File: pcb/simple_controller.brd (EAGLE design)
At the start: 40 x 52 mm, 66 parts, among them IC1 LD1117S50C, IC2 ST2378E, IC3 MCP1802, IC4 INA196, IC5 INA196, IC6 ATSAMC21G, Q1 24MHz, Q2 32768kHz, T1 NVR4003NT3G, T2 IRF9392PBF, T3 NVR4003NT3G, T4 IRF9392PBF, X1 NANOFIT-2, X11 PINHD-1X2, X2 IGRID-14, X3 IGRID-10, X4 PINHD-1X2, X5 MICRO-LATCH-4, X6 PINHD-1X2, X7 NANOFIT-7, X8 JTAG-EDGE-CON, X9 B3S-1000

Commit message: fixing op amp (iron,tweezer)
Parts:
- C2, C3, C4, C5: value 10µF -> 1µF
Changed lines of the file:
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@@
 <grid distance="0.4" unitdist="mm" unit="mm" style="lines" multiple="1" display="no" altdistance="0.05" altunitdist="mm" altunit="mm"/>
 <layers>
-<layer number="1" name="Top" color="4" fill="1" visible="yes" active="yes"/>
+<layer number="1" name="Top" color="4" fill="1" visible="no" active="yes"/>
 <layer number="2" name="Route2" color="1" fill="3" visible="no" active="no"/>
 <layer number="3" name="Route3" color="4" fill="3" visible="no" active="no"/>
@@
 <layer number="19" name="Unrouted" color="6" fill="1" visible="yes" active="yes"/>
 <layer number="20" name="Dimension" color="24" fill="1" visible="yes" active="yes"/>
-<layer number="21" name="tPlace" color="7" fill="1" visible="yes" active="yes"/>
+<layer number="21" name="tPlace" color="7" fill="1" visible="no" active="yes"/>
 <layer number="22" name="bPlace" color="7" fill="1" visible="yes" active="yes"/>
-<layer number="23" name="tOrigins" color="15" fill="1" visible="yes" active="yes"/>
+<layer number="23" name="tOrigins" color="15" fill="1" visible="no" active="yes"/>
 <layer number="24" name="bOrigins" color="15" fill="1" visible="yes" active="yes"/>
-<layer number="25" name="tNames" color="7" fill="1" visible="yes" active="yes"/>
-<layer number="26" name="bNames" color="7" fill="1" visible="yes" active="yes"/>
+<layer number="25" name="tNames" color="7" fill="1" visible="no" active="yes"/>
+<layer number="26" name="bNames" color="7" fill="1" visible="no" active="yes"/>
 <layer number="27" name="tValues" color="7" fill="1" visible="no" active="yes"/>
 <layer number="28" name="bValues" color="7" fill="1" visible="no" active="yes"/>
@@
 <layer number="37" name="tTest" color="7" fill="1" visible="no" active="yes"/>
 <layer number="38" name="bTest" color="7" fill="1" visible="no" active="yes"/>
-<layer number="39" name="tKeepout" color="4" fill="11" visible="yes" active="yes"/>
-<layer number="40" name="bKeepout" color="1" fill="11" visible="yes" active="yes"/>
-<layer number="41" name="tRestrict" color="4" fill="10" visible="yes" active="yes"/>
-<layer number="42" name="bRestrict" color="1" fill="10" visible="yes" active="yes"/>
-<layer number="43" name="vRestrict" color="2" fill="10" visible="yes" active="yes"/>
+<layer number="39" name="tKeepout" color="4" fill="11" visible="no" active="yes"/>
+<layer number="40" name="bKeepout" color="1" fill="11" visible="no" active="yes"/>
+<layer number="41" name="tRestrict" color="4" fill="10" visible="no" active="yes"/>
+<layer number="42" name="bRestrict" color="1" fill="10" visible="no" active="yes"/>
+<layer number="43" name="vRestrict" color="2" fill="10" visible="no" active="yes"/>
 <layer number="44" name="Drills" color="7" fill="1" visible="no" active="yes"/>
 <layer number="45" name="Holes" color="7" fill="1" visible="yes" active="yes"/>
@@
 <layer number="48" name="Document" color="7" fill="1" visible="no" active="yes"/>
 <layer number="49" name="Reference" color="7" fill="1" visible="no" active="yes"/>
-<layer number="51" name="tDocu" color="7" fill="1" visible="yes" active="yes"/>
+<layer number="51" name="tDocu" color="7" fill="1" visible="no" active="yes"/>
 <layer number="52" name="bDocu" color="7" fill="1" visible="yes" active="yes"/>
 <layer number="88" name="SimResults" color="9" fill="1" visible="no" active="no"/>
@@
 <attribute name="OC_MOUSER" value="667-EEE-FK1E471P" x="8.5" y="22.7" size="1.778" layer="27" rot="R180" display="off"/>
 </element>
-<element name="C2" library="rcl" library_urn="urn:adsk.eagle:library:334" package="C0805" package3d_urn="urn:adsk.eagle:package:23617/2" value="10µF" x="2.6" y="36.65" smashed="yes" rot="MR0">
+<element name="C2" library="rcl" library_urn="urn:adsk.eagle:library:334" package="C0805" package3d_urn="urn:adsk.eagle:package:23617/2" value="1µF" x="2.6" y="36.65" smashed="yes" rot="MR0">
 <attribute name="NAME" x="3.148665625" y="37.7854" size="0.8128" layer="26" rot="MR0"/>
 <attribute name="OC_MOUSER" value="81-GRM21BR61E106MA3L" x="2.6" y="36.65" size="1.778" layer="28" rot="MR0" display="off"/>
@@
 <attribute name="VALUE" x="3.87" y="34.11" size="1.27" layer="28" rot="MR0"/>
 </element>
-<element name="C3" library="rcl" library_urn="urn:adsk.eagle:library:334" package="C0805" package3d_urn="urn:adsk.eagle:package:23617/2" value="10µF" x="3.8" y="23.15" smashed="yes" rot="MR0">
+<element name="C3" library="rcl" library_urn="urn:adsk.eagle:library:334" package="C0805" package3d_urn="urn:adsk.eagle:package:23617/2" value="1µF" x="3.8" y="23.15" smashed="yes" rot="MR0">
 <attribute name="NAME" x="1.8016" y="22.7436" size="0.8128" layer="26" rot="MR0"/>
 <attribute name="OC_MOUSER" value="81-GRM21BR61E106MA3L" x="3.8" y="23.15" size="1.778" layer="28" rot="MR0" display="off"/>
@@
 <attribute name="VALUE" x="5.07" y="20.61" size="1.27" layer="28" rot="MR0"/>
 </element>
-<element name="C4" library="rcl" library_urn="urn:adsk.eagle:library:334" package="C0805" package3d_urn="urn:adsk.eagle:package:23617/2" value="10µF" x="3.8" y="21.1" smashed="yes" rot="MR0">
+<element name="C4" library="rcl" library_urn="urn:adsk.eagle:library:334" package="C0805" package3d_urn="urn:adsk.eagle:package:23617/2" value="1µF" x="3.8" y="21.1" smashed="yes" rot="MR0">
 <attribute name="NAME" x="1.8016" y="20.6936" size="0.8128" layer="26" rot="MR0"/>
 <attribute name="OC_MOUSER" value="81-GRM21BR61E106MA3L" x="3.8" y="21.1" size="1.778" layer="28" rot="MR0" display="off"/>
@@
 <attribute name="VALUE" x="5.07" y="18.56" size="1.27" layer="28" rot="MR0"/>
 </element>
-<element name="C5" library="rcl" library_urn="urn:adsk.eagle:library:334" package="C0805" package3d_urn="urn:adsk.eagle:package:23617/2" value="10µF" x="2.85" y="13.4" smashed="yes" rot="MR180">
+<element name="C5" library="rcl" library_urn="urn:adsk.eagle:library:334" package="C0805" package3d_urn="urn:adsk.eagle:package:23617/2" value="1µF" x="2.85" y="13.4" smashed="yes" rot="MR180">
 <attribute name="NAME" x="1.948928125" y="11.4518" size="0.8128" layer="26" rot="MR0"/>
 <attribute name="OC_MOUSER" value="81-GRM21BR61E106MA3L" x="2.85" y="13.4" size="1.778" layer="28" rot="MR180" display="off"/>

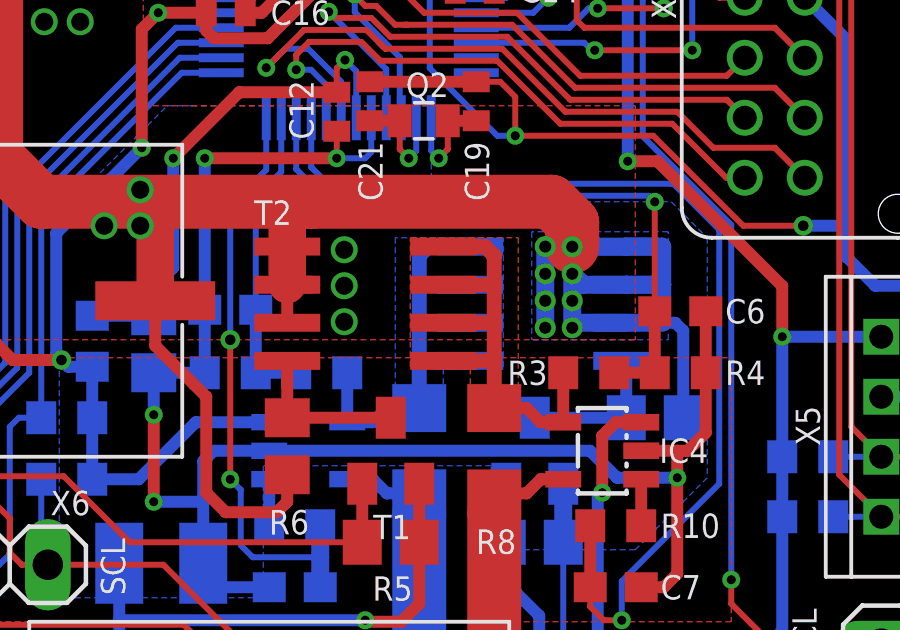
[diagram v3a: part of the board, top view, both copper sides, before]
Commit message: iron drills deleted
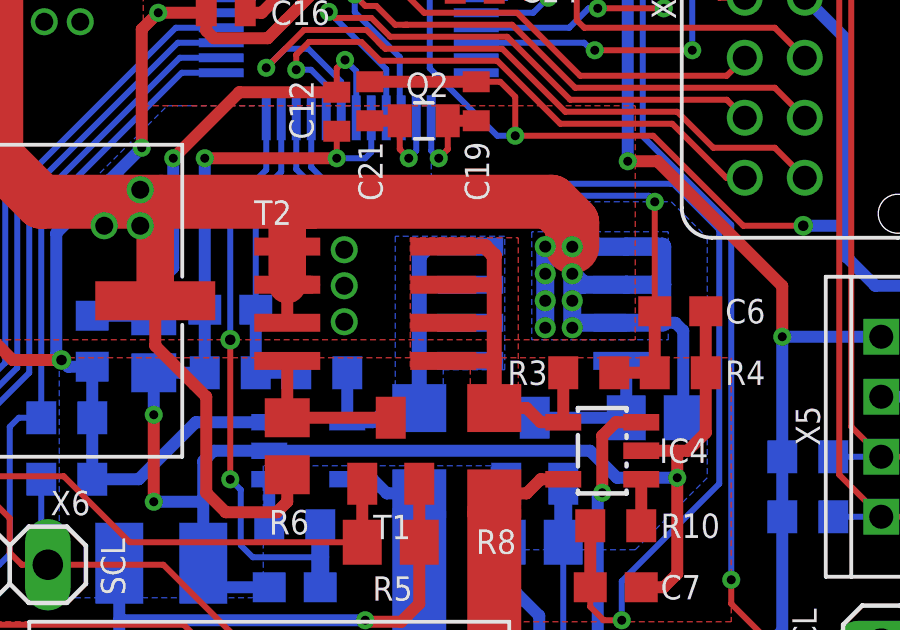
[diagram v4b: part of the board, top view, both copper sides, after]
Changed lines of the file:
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@@
 <grid distance="1" unitdist="mm" unit="mm" style="lines" multiple="1" display="no" altdistance="0.05" altunitdist="mm" altunit="mm"/>
 <layers>
-<layer number="1" name="Top" color="4" fill="1" visible="yes" active="yes"/>
+<layer number="1" name="Top" color="4" fill="1" visible="no" active="yes"/>
 <layer number="2" name="Route2" color="1" fill="3" visible="no" active="no"/>
 <layer number="3" name="Route3" color="4" fill="3" visible="no" active="no"/>
@@
 <layer number="19" name="Unrouted" color="6" fill="1" visible="yes" active="yes"/>
 <layer number="20" name="Dimension" color="24" fill="1" visible="yes" active="yes"/>
-<layer number="21" name="tPlace" color="7" fill="1" visible="yes" active="yes"/>
+<layer number="21" name="tPlace" color="7" fill="1" visible="no" active="yes"/>
 <layer number="22" name="bPlace" color="7" fill="1" visible="yes" active="yes"/>
-<layer number="23" name="tOrigins" color="15" fill="1" visible="yes" active="yes"/>
+<layer number="23" name="tOrigins" color="15" fill="1" visible="no" active="yes"/>
 <layer number="24" name="bOrigins" color="15" fill="1" visible="yes" active="yes"/>
 <layer number="25" name="tNames" color="7" fill="1" visible="no" active="yes"/>
@@
 <layer number="37" name="tTest" color="7" fill="1" visible="no" active="yes"/>
 <layer number="38" name="bTest" color="7" fill="1" visible="no" active="yes"/>
-<layer number="39" name="tKeepout" color="4" fill="11" visible="yes" active="yes"/>
+<layer number="39" name="tKeepout" color="4" fill="11" visible="no" active="yes"/>
 <layer number="40" name="bKeepout" color="1" fill="11" visible="yes" active="yes"/>
 <layer number="41" name="tRestrict" color="4" fill="10" visible="no" active="yes"/>
@@
 <wire x1="21.95" y1="30.45" x2="24.2" y2="28.2" width="0.2" layer="16"/>
 <wire x1="29.4" y1="28.2" x2="24.8" y2="28.2" width="0.2" layer="1"/>
-<polygon width="0.2" layer="16" isolate="0.3048" rank="3">
+<polygon width="0" layer="16" isolate="0.3048" rank="3">
 <vertex x="0" y="52"/>
 <vertex x="40" y="52"/>
@@
 <wire x1="21.6" y1="24.2" x2="21.905" y2="24.505" width="0.5" layer="16"/>
 <wire x1="21.6" y1="24.2" x2="21.6" y2="23.235" width="0.5" layer="16"/>
-<polygon width="0.2" layer="16" thermals="no">
-<vertex x="20.8" y="24.8"/>
+<polygon width="0" layer="16" thermals="no">
+<vertex x="20.8" y="24.85"/>
 <vertex x="20.8" y="19.6"/>
 <vertex x="22.4" y="19.6"/>
-<vertex x="22.4" y="20.5"/>
-<vertex x="24.4" y="20.5"/>
-<vertex x="24.4" y="24.8"/>
+<vertex x="22.4" y="20.4"/>
+<vertex x="24.45" y="20.4"/>
+<vertex x="24.45" y="24.85"/>
 </polygon>
 </signal>
@@
 <contactref element="T2" pad="1"/>
 <wire x1="17.2" y1="23.235" x2="18" y2="23.235" width="0.6" layer="1"/>
-<polygon width="0.2" layer="16" isolate="0.3048" thermals="no">
+<polygon width="0" layer="16" isolate="0.3048" thermals="no">
 <vertex x="25.35" y="21.4"/>
 <vertex x="29.9" y="21.4"/>
